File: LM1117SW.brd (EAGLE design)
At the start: 160 x 100 mm, 7 parts

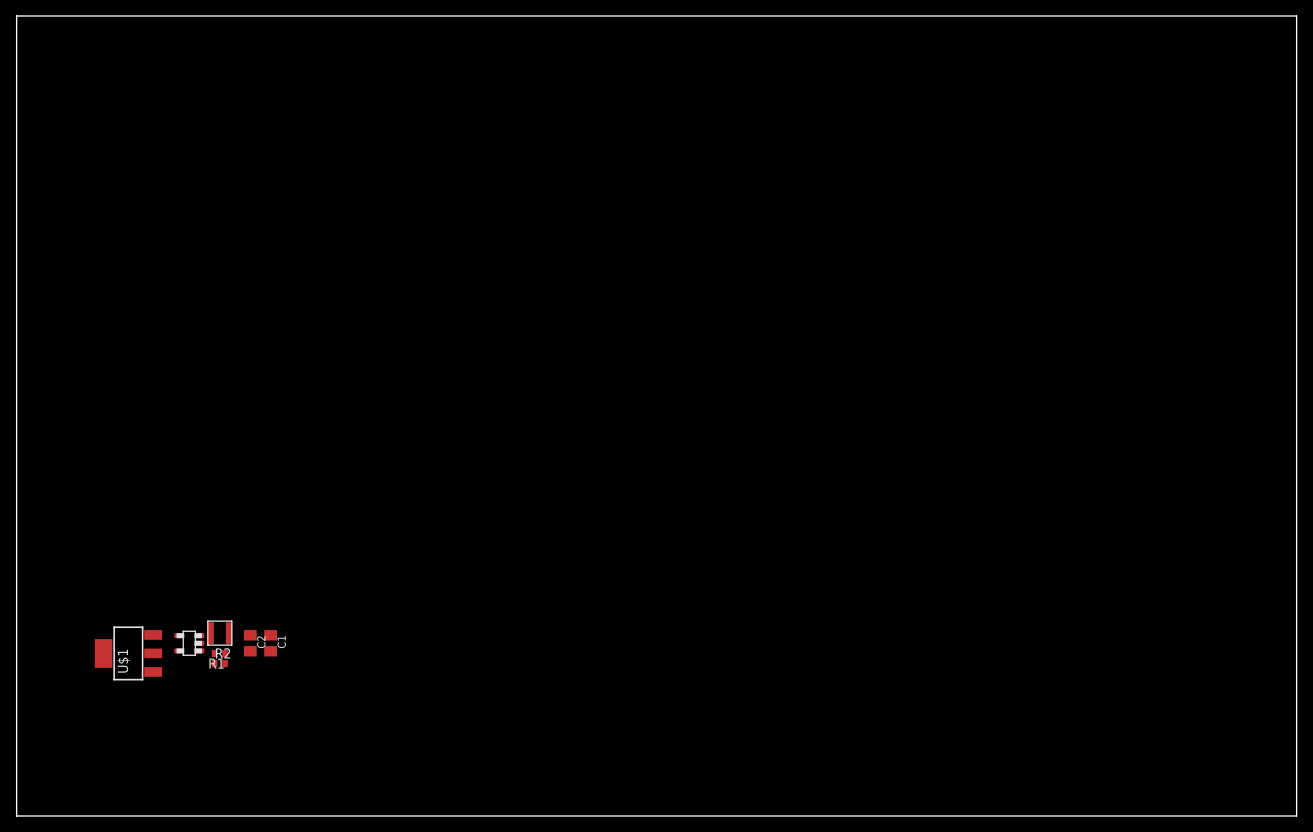
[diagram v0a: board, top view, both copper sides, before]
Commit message: layout stuff
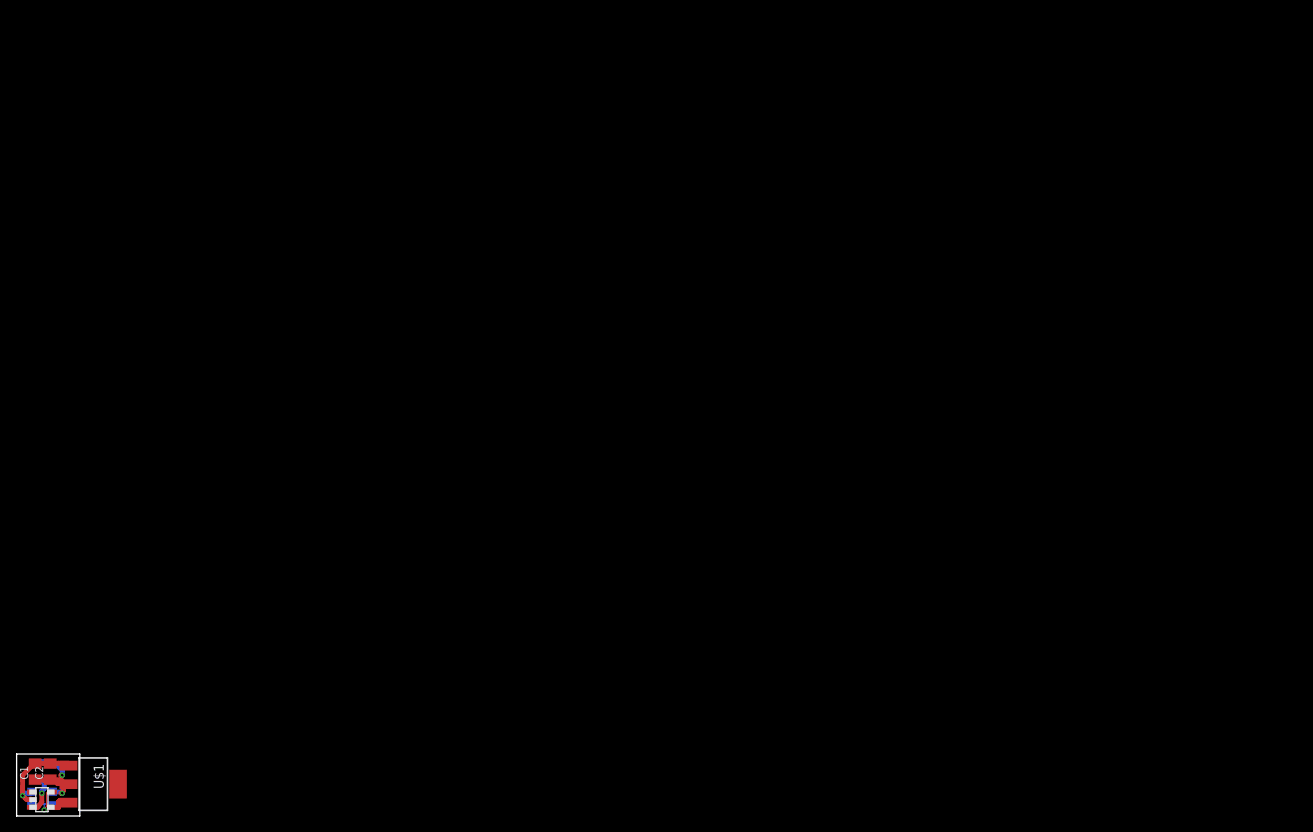
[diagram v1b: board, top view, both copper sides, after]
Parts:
- R1, R2: device rcl:R0402 -> rcl:R0603
- moved C1 33.5 mm to (2.32, 5.55), turned to 90 degrees
- moved C2 29.7 mm to (4.20, 5.55), turned to 90 degrees
- moved R2 28.9 mm to (1.89, 2.18), flipped to the bottom, turned to 90 degrees
- moved L1 27.9 mm to (3.55, 5.56), flipped to the bottom, turned to 90 degrees
- moved R1 27.7 mm to (4.50, 2.19), flipped to the bottom, turned to 270 degrees
- moved U$2 26.9 mm to (3.16, 2.04), turned to 270 degrees
- moved U$1 16.9 mm to (9.58, 3.98), turned to 270 degrees
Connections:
- net N$2 renamed VOUT
- net N$3 renamed SENS
- net N$4 renamed VIN
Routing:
- net VOUT: track 0.00 -> 12.9 mm, vias 0 -> 2
- net GND: track 0.00 -> 11.9 mm, vias 0 -> 1
- net SENS: track 0.00 -> 6.60 mm, vias 0 -> 1
- net N$1: track 0.00 -> 5.70 mm, vias 0 -> 1
- net VIN: track 0.00 -> 3.04 mm
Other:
- board size 160 x 100 mm -> 7.9 x 7.8 mm
